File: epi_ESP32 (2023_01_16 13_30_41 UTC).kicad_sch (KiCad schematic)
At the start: 35 parts, among them J1 Conn_01x08, J2 Conn_01x08, J3 USB_C_Receptacle_USB2.0, SW1 SW_MEC_5G, SW2 SW_MEC_5G, U1 ESP32-C3, U2 RT9080, Y1 Crystal_GND24

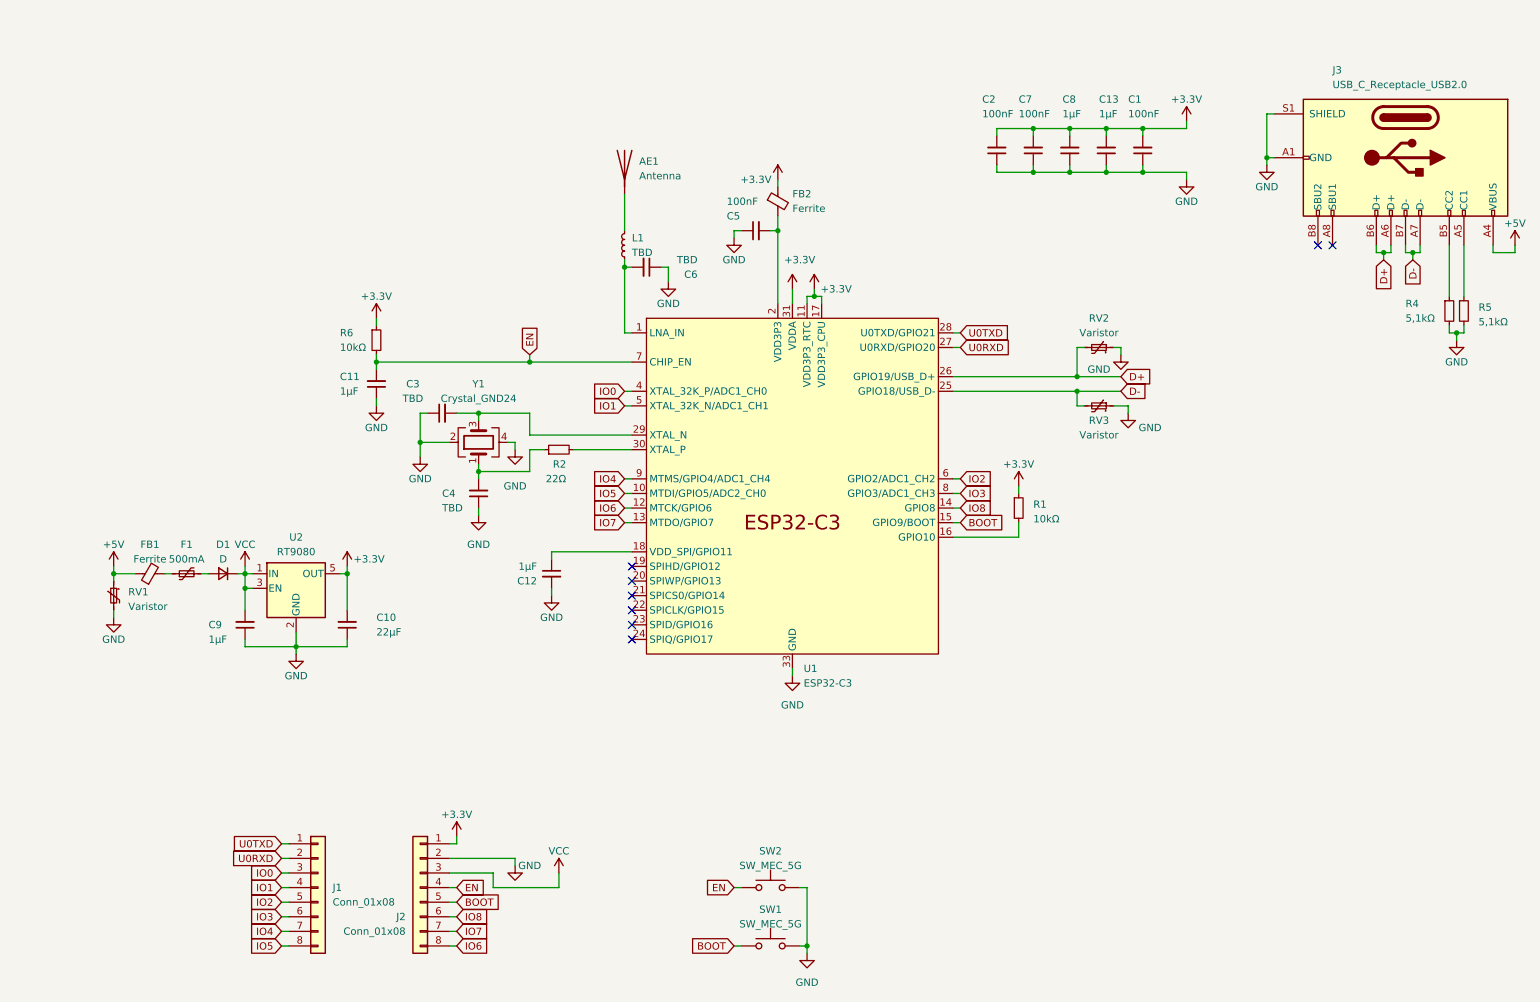
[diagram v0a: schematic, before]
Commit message: pictures and schematic
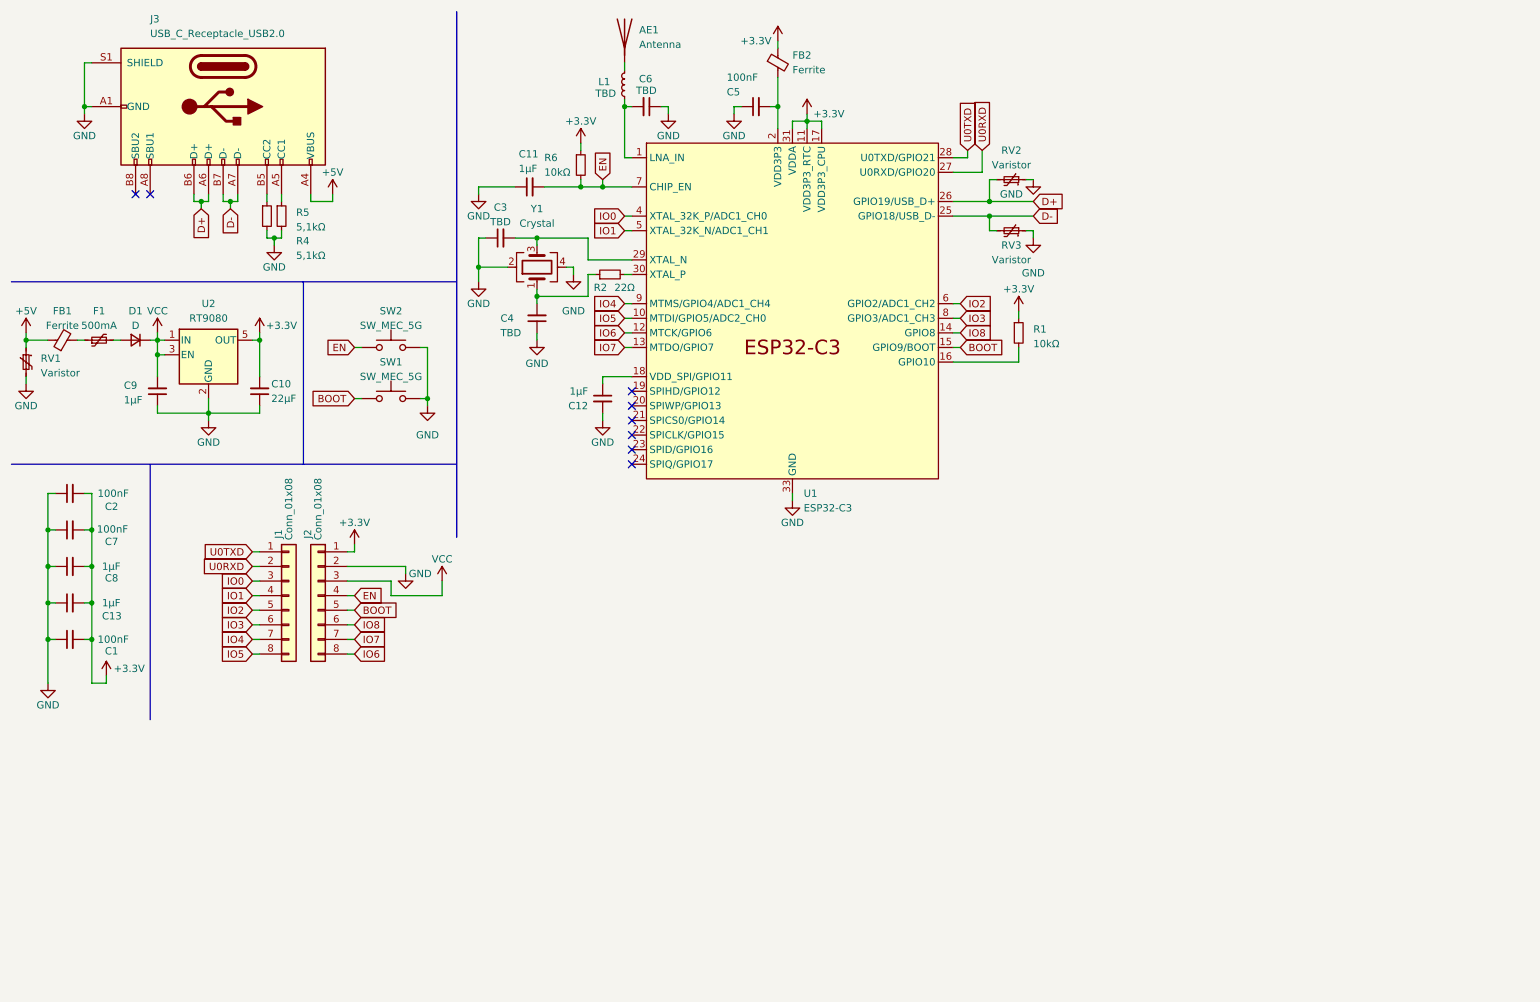
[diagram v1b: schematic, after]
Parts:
- Y1: value Crystal_GND24 -> Crystal
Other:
- company: (none) -> Ping hobbyelektronik
- title: (none) -> Epi C3
- moved on the sheet: AE1, C1, C10, C11, C12, C13, C2, C3, C4, C5, C6, C7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

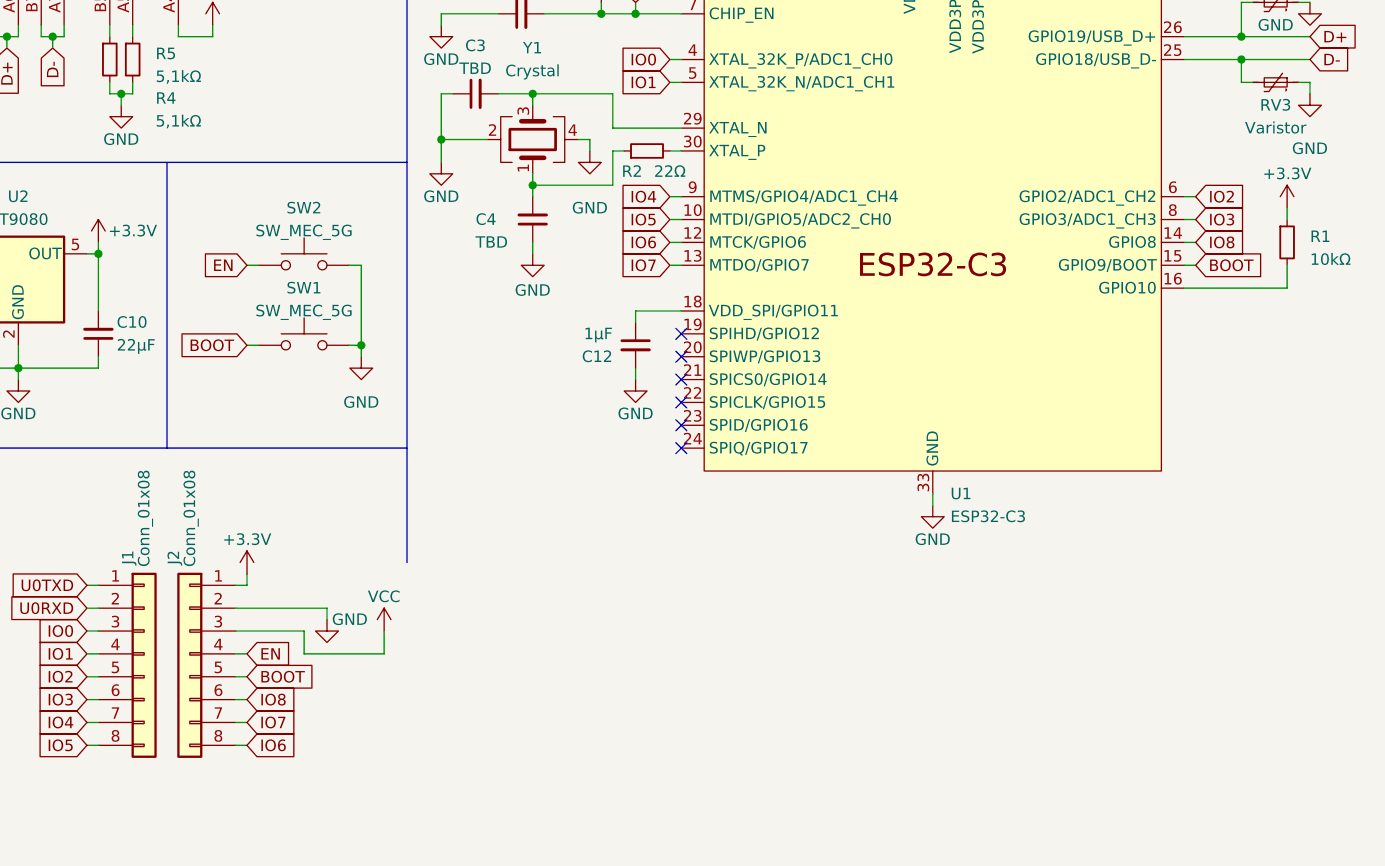
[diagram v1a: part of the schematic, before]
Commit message: new revision
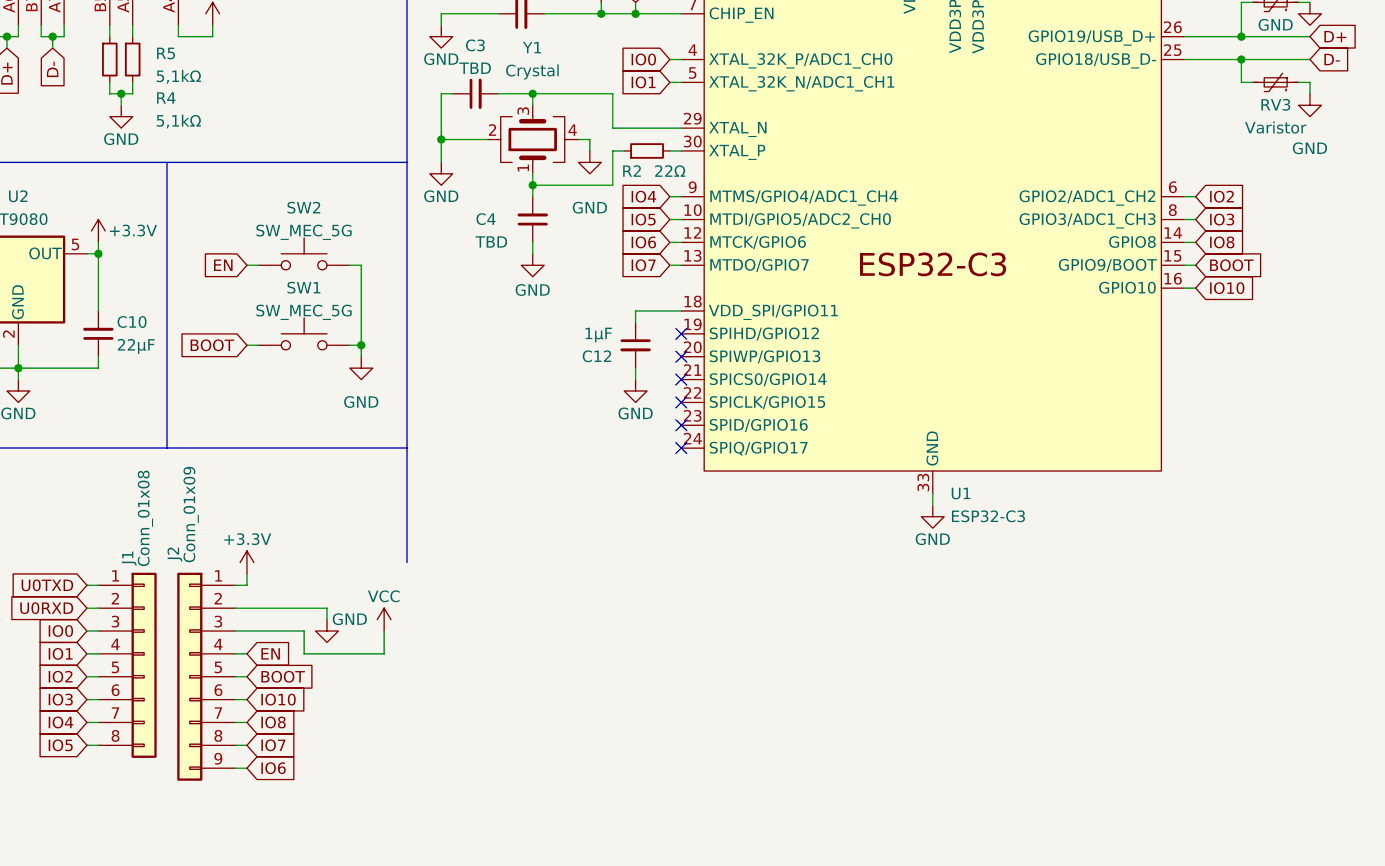
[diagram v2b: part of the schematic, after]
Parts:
- removed J2: Conn_01x08, Connector_PinHeader_1.27mm:PinHeader_1x08_P1.27mm_Vertical, symbol Connector_Generic:Conn_01x08
- removed R1: 10kΩ, Resistor_SMD:R_0402_1005Metric, symbol Device:R_Small
- added J2: Conn_01x09, Connector_PinSocket_1.27mm:PinSocket_1x09_P1.27mm_Vertical, symbol Connector_Generic:Conn_01x09
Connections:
- net +3.3V: now also J2.1 (Pin_1)
- net BOOT: now also J2.5 (Pin_5)
- net EN: now also J2.4 (Pin_4)
- net GND: now also J2.2 (Pin_2)
- net IO6: now also J2.9 (Pin_9)
- net IO7: now also J2.8 (Pin_8)
- net IO8: now also J2.7 (Pin_7)
- net VCC: now also J2.3 (Pin_3)
- net IO10: now reaches U1.16 (GPIO10)
- net IO10: now also J2.6 (Pin_6)
